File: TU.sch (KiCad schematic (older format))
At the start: 6 parts, among them J1 Conn_01x06_Male, J2 Conn_01x17_Male, J3 Conn_Coaxial, J4 Debugger, J7 Conn_Coaxial, SW1 SW_DPST_x2

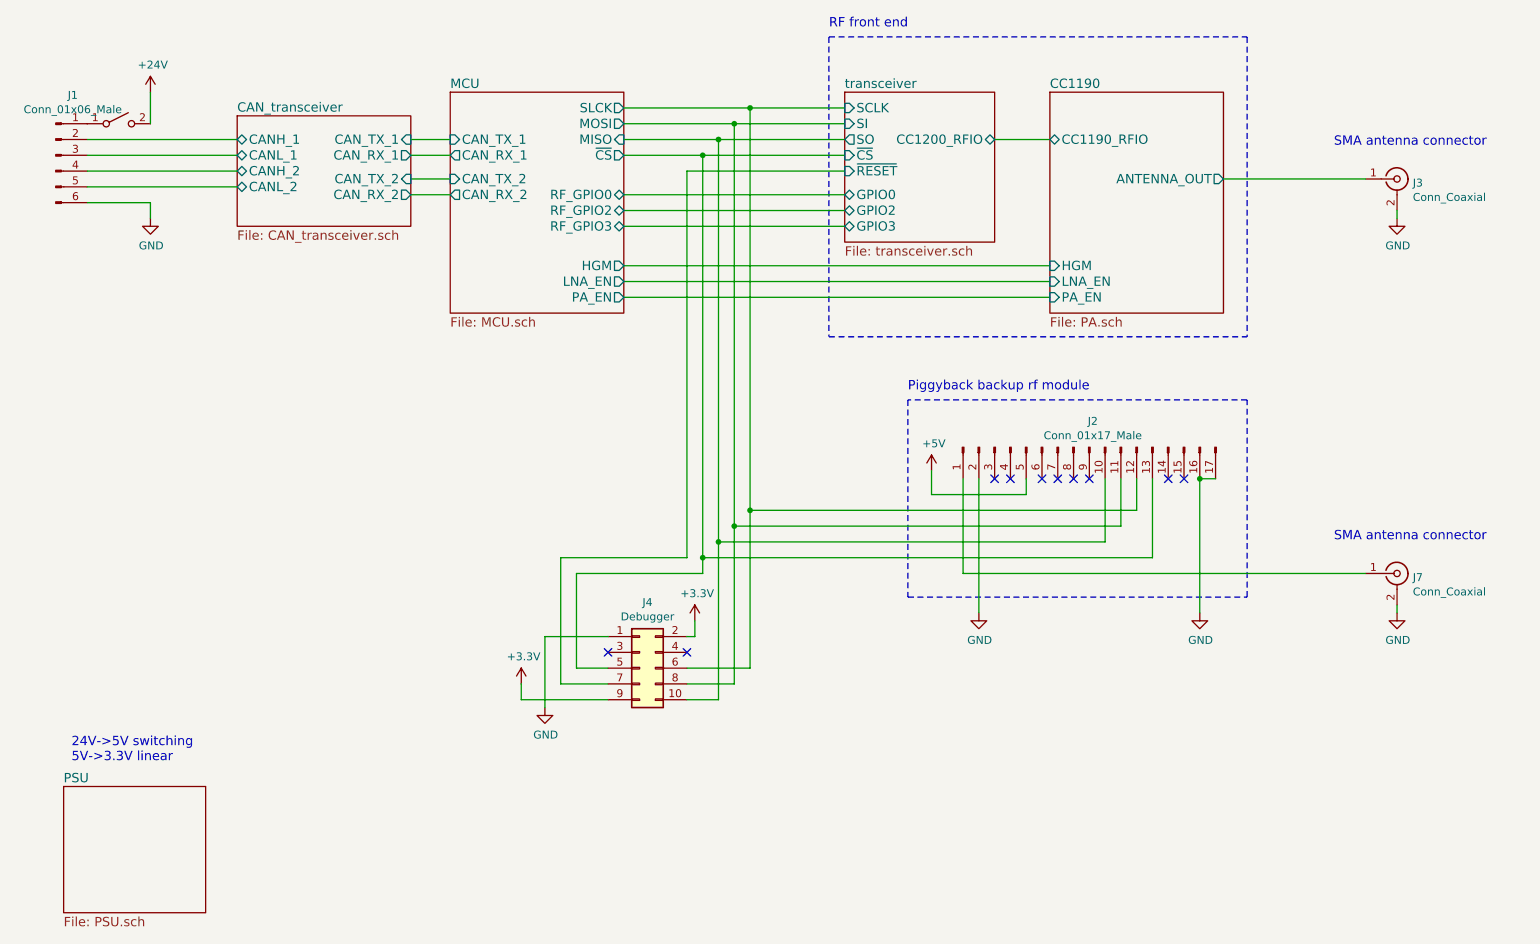
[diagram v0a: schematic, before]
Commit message: Small changes to schematic
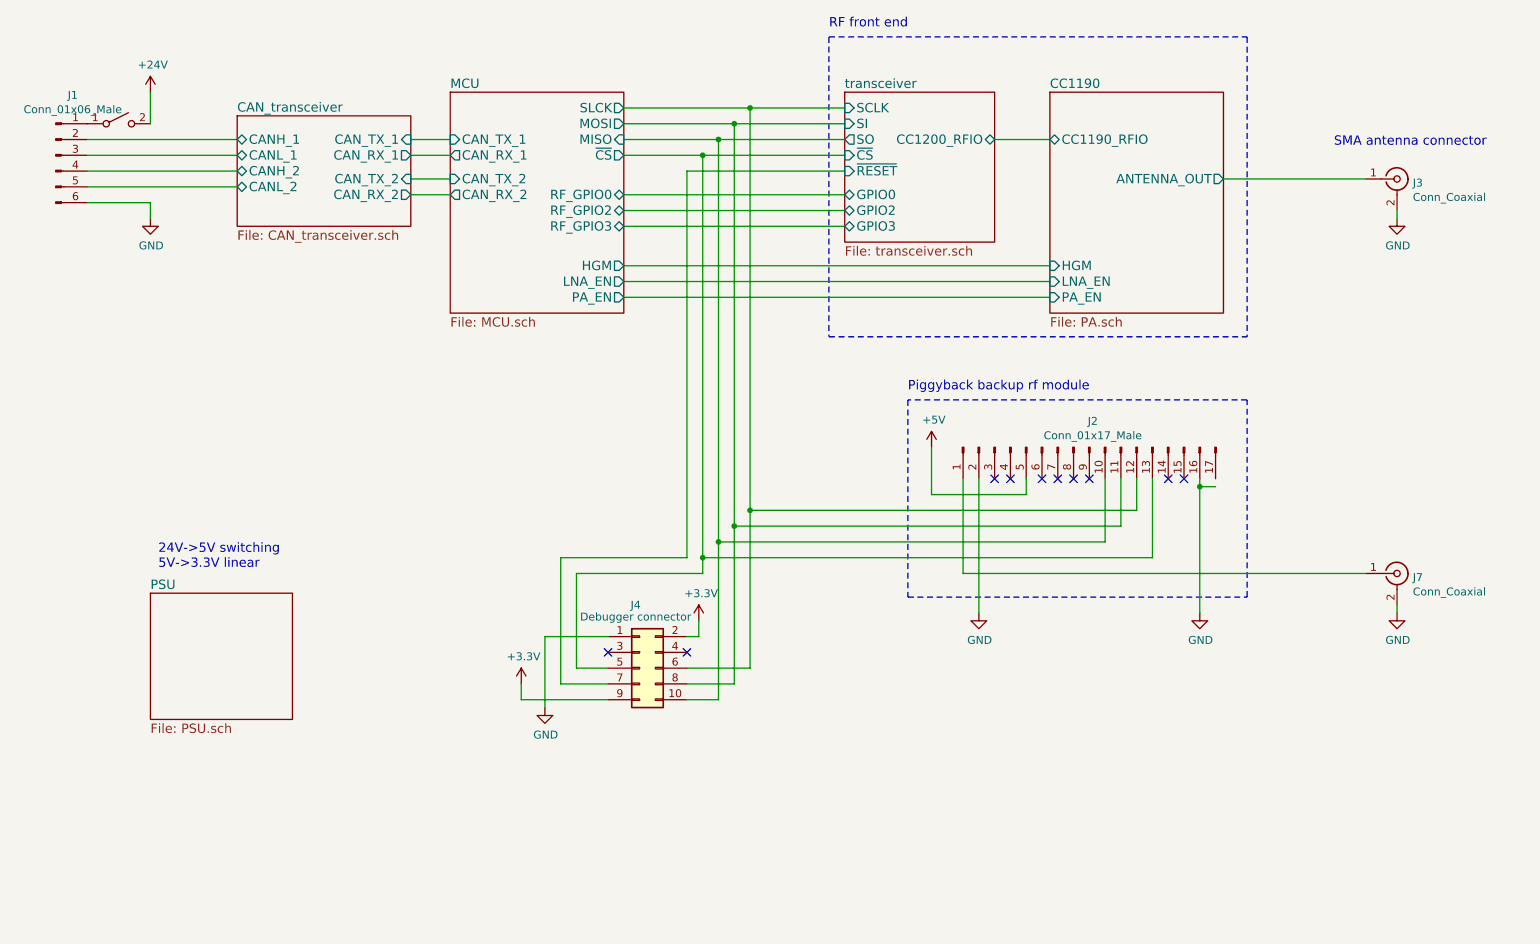
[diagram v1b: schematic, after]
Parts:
- J4: value Debugger -> Debugger connector
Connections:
- net GND: no longer J2.17 (Pin_17)
